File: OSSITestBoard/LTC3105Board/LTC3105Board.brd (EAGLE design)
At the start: 20.3 x 22.9 mm, 20 parts, among them U1 LT3105-MS

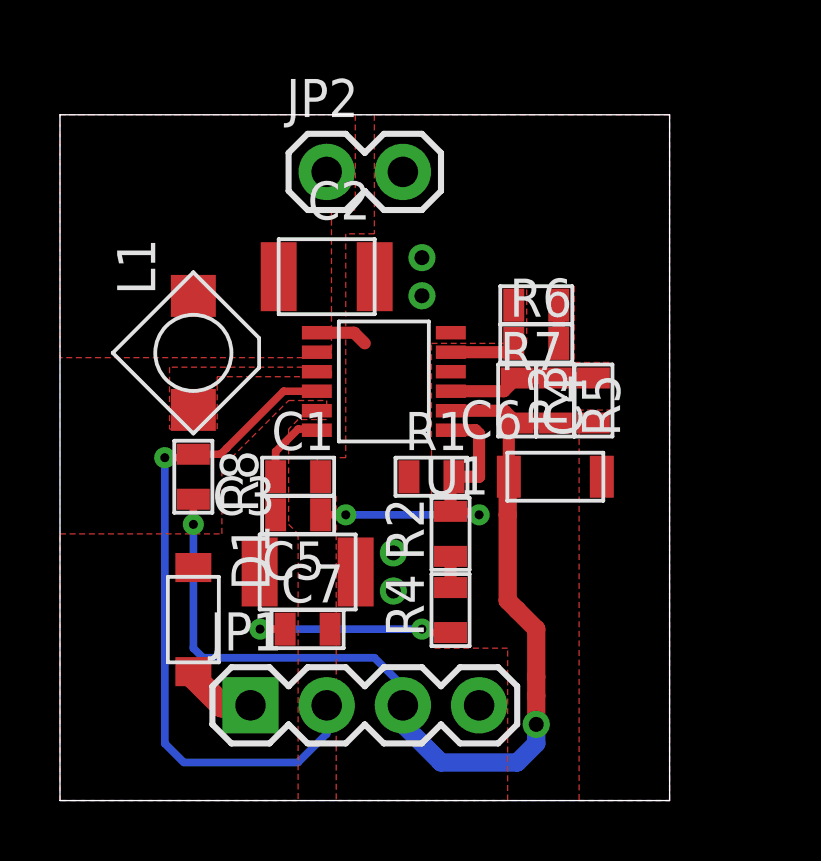
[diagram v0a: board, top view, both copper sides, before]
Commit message: LTC3105 board notes added
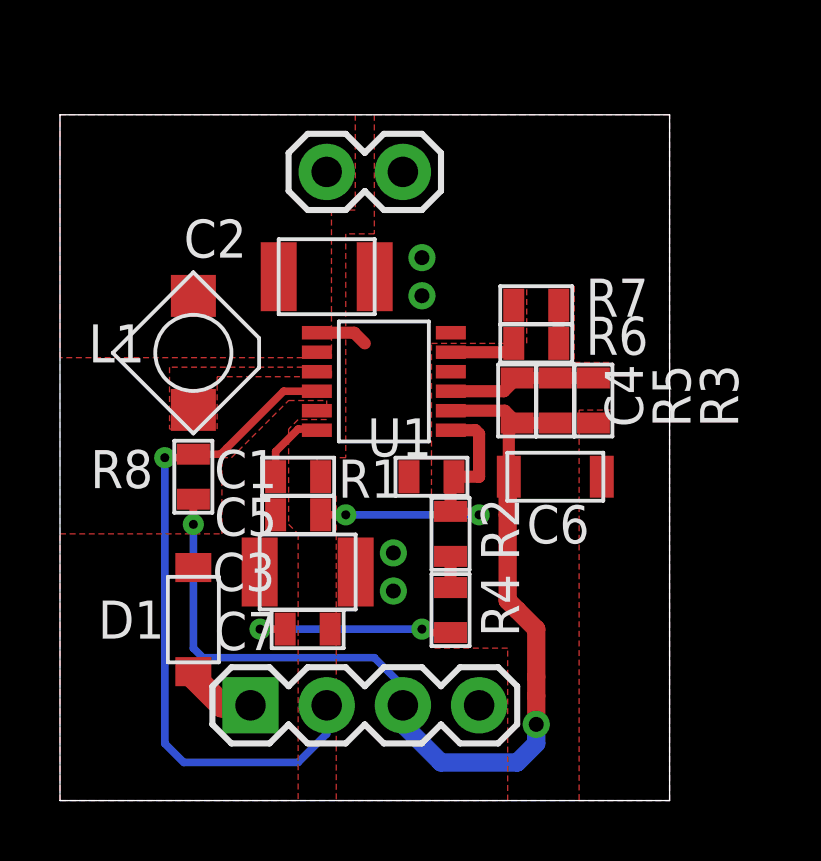
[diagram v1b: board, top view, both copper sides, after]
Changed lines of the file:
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@@
 <layer number="19" name="Unrouted" color="6" fill="1" visible="yes" active="yes"/>
 <layer number="20" name="Dimension" color="15" fill="1" visible="yes" active="yes"/>
-<layer number="21" name="tPlace" color="7" fill="1" visible="yes" active="yes"/>
+<layer number="21" name="tPlace" color="7" fill="1" visible="no" active="yes"/>
 <layer number="22" name="bPlace" color="7" fill="1" visible="no" active="yes"/>
-<layer number="23" name="tOrigins" color="15" fill="1" visible="yes" active="yes"/>
-<layer number="24" name="bOrigins" color="15" fill="1" visible="yes" active="yes"/>
-<layer number="25" name="tNames" color="7" fill="1" visible="no" active="yes"/>
-<layer number="26" name="bNames" color="7" fill="1" visible="no" active="yes"/>
+<layer number="23" name="tOrigins" color="15" fill="1" visible="no" active="yes"/>
+<layer number="24" name="bOrigins" color="15" fill="1" visible="no" active="yes"/>
+<layer number="25" name="tNames" color="7" fill="1" visible="yes" active="yes"/>
+<layer number="26" name="bNames" color="7" fill="1" visible="yes" active="yes"/>
 <layer number="27" name="tValues" color="7" fill="1" visible="no" active="yes"/>
 <layer number="28" name="bValues" color="7" fill="1" visible="no" active="yes"/>
-<layer number="29" name="tStop" color="7" fill="3" visible="yes" active="yes"/>
-<layer number="30" name="bStop" color="7" fill="6" visible="yes" active="yes"/>
+<layer number="29" name="tStop" color="7" fill="3" visible="no" active="yes"/>
+<layer number="30" name="bStop" color="7" fill="6" visible="no" active="yes"/>
 <layer number="31" name="tCream" color="7" fill="4" visible="no" active="yes"/>
 <layer number="32" name="bCream" color="7" fill="5" visible="no" active="yes"/>
@@
 <rectangle x1="0" y1="-1.27" x2="20.32" y2="21.59" layer="29"/>
 <rectangle x1="0" y1="-1.27" x2="20.32" y2="21.59" layer="30"/>
+<circle x="12.7" y="10.16" radius="0.3175" width="0.254" layer="48"/>
 </plain>
 <attributes>
@@
 <elements>
 <element name="U1" library="OSSI" package="MSOP-12-MS" value="LT3105-MS" x="10.795" y="12.7" smashed="yes" rot="R90">
-<attribute name="NAME" x="14.295" y="10.2" size="1.27" layer="25" font="vector" rot="R180"/>
+<attribute name="NAME" x="12.39" y="11.47" size="1.27" layer="25" font="vector" rot="R180"/>
 <attribute name="VALUE" x="14.295" y="16.2" size="1.27" layer="27" rot="R180"/>
 </element>
 <element name="L1" library="OSSI" package="CDRH3D18" value="10uH" x="4.445" y="13.6525" smashed="yes" rot="R270">
-<attribute name="NAME" x="1.905" y="17.4625" size="1.27" layer="25" font="vector" rot="R270"/>
+<attribute name="NAME" x="0.9525" y="13.335" size="1.27" layer="25" font="vector"/>
 <attribute name="VALUE" x="-3.175" y="16.1925" size="1.27" layer="27" rot="R270"/>
 </element>
 <element name="C1" library="OSSI" package="C0603(1608)" value="1uF" x="7.9375" y="9.525" smashed="yes">
-<attribute name="NAME" x="7.0485" y="10.414" size="1.27" layer="25" font="vector"/>
+<attribute name="NAME" x="5.1435" y="9.144" size="1.27" layer="25" font="vector"/>
 <attribute name="VALUE" x="7.0485" y="7.493" size="1.27" layer="27"/>
 </element>
 <element name="C2" library="OSSI" package="C1210-GCM32" value="10uF, 1210" x="8.89" y="16.1925" smashed="yes">
-<attribute name="NAME" x="8.255" y="18.0975" size="1.27" layer="25" font="vector"/>
+<attribute name="NAME" x="4.1275" y="16.8275" size="1.27" layer="25" font="vector"/>
 <attribute name="VALUE" x="5.715" y="13.0175" size="1.27" layer="27"/>
 </element>
 <element name="R1" library="OSSI" package="R0603(1608)" value="499k, 1%" x="12.3825" y="9.525" smashed="yes">
-<attribute name="NAME" x="11.4935" y="10.414" size="1.27" layer="25" font="vector"/>
+<attribute name="NAME" x="9.271" y="8.8265" size="1.27" layer="25" font="vector"/>
 <attribute name="VALUE" x="11.4935" y="7.493" size="1.27" layer="27"/>
 </element>
 <element name="R2" library="OSSI" package="R0603(1608)" value="392k, 1%" x="13.0175" y="7.62" smashed="yes" rot="R90">
-<attribute name="NAME" x="12.1285" y="6.731" size="1.27" layer="25" font="vector" rot="R90"/>
+<attribute name="NAME" x="15.3035" y="6.731" size="1.27" layer="25" font="vector" rot="R90"/>
 <attribute name="VALUE" x="15.0495" y="6.731" size="1.27" layer="27" rot="R90"/>
 </element>
 <element name="C4" library="OSSI" package="C0603(1608)" value="33pF" x="15.24" y="12.065" smashed="yes" rot="R270">
-<attribute name="NAME" x="16.129" y="12.954" size="1.27" layer="25" font="vector" rot="R270"/>
+<attribute name="NAME" x="19.431" y="11.176" size="1.27" layer="25" font="vector" rot="R90"/>
 <attribute name="VALUE" x="13.208" y="12.954" size="1.27" layer="27" rot="R270"/>
 </element>
 <element name="R3" library="OSSI" package="R0603(1608)" value="549k, 1%" x="17.78" y="12.065" smashed="yes" rot="R90">
-<attribute name="NAME" x="16.891" y="11.176" size="1.27" layer="25" font="vector" rot="R90"/>
+<attribute name="NAME" x="22.606" y="11.176" size="1.27" layer="25" font="vector" rot="R90"/>
 <attribute name="VALUE" x="19.812" y="11.176" size="1.27" layer="27" rot="R90"/>
 </element>
 <element name="R4" library="OSSI" package="R0603(1608)" value="750k, 1%" x="13.0175" y="5.08" smashed="yes" rot="R90">
-<attribute name="NAME" x="12.1285" y="4.191" size="1.27" layer="25" font="vector" rot="R90"/>
+<attribute name="NAME" x="15.3035" y="4.191" size="1.27" layer="25" font="vector" rot="R90"/>
 <attribute name="VALUE" x="15.0495" y="4.191" size="1.27" layer="27" rot="R90"/>
 </element>
 <element name="C5" library="OSSI" package="C0603(1608)" value="33pF" x="7.9375" y="8.255" smashed="yes" rot="R180">
-<attribute name="NAME" x="8.8265" y="7.366" size="1.27" layer="25" font="vector" rot="R180"/>
+<attribute name="NAME" x="5.1435" y="7.5565" size="1.27" layer="25" font="vector"/>
 <attribute name="VALUE" x="8.8265" y="10.287" size="1.27" layer="27" rot="R180"/>
 </element>
 <element name="R5" library="OSSI" package="R0603(1608)" value="1.1M, 1%" x="16.51" y="12.065" smashed="yes" rot="R270">
-<attribute name="NAME" x="17.399" y="12.954" size="1.27" layer="25" font="vector" rot="R270"/>
+<attribute name="NAME" x="21.0185" y="11.176" size="1.27" layer="25" font="vector" rot="R90"/>
 <attribute name="VALUE" x="14.478" y="12.954" size="1.27" layer="27" rot="R270"/>
 </element>
 <element name="R6" library="OSSI" package="R0603(1608)" value="TBD" x="15.875" y="13.97" smashed="yes">
-<attribute name="NAME" x="14.986" y="14.859" size="1.27" layer="25" font="vector"/>
+<attribute name="NAME" x="17.526" y="13.589" size="1.27" layer="25" font="vector"/>
 <attribute name="VALUE" x="14.986" y="11.938" size="1.27" layer="27"/>
 </element>
 <element name="R7" library="OSSI" package="R0603(1608)" value="TBD" x="15.875" y="15.24" smashed="yes" rot="R180">
-<attribute name="NAME" x="16.764" y="14.351" size="1.27" layer="25" font="vector" rot="R180"/>
+<attribute name="NAME" x="17.526" y="14.859" size="1.27" layer="25" font="vector"/>
 <attribute name="VALUE" x="16.764" y="17.272" size="1.27" layer="27" rot="R180"/>
 </element>
 <element name="R8" library="OSSI" package="R0603(1608)" value="100k" x="4.445" y="9.525" smashed="yes" rot="R270">
-<attribute name="NAME" x="5.334" y="10.414" size="1.27" layer="25" font="vector" rot="R270"/>
+<attribute name="NAME" x="1.016" y="9.144" size="1.27" layer="25" font="vector"/>
 <attribute name="VALUE" x="2.413" y="10.414" size="1.27" layer="27" rot="R270"/>
 </element>
 <element name="C6" library="OSSI" package="C1206-GCM31" value="4.7uF, 1206" x="16.51" y="9.525" smashed="yes">
-<attribute name="NAME" x="13.335" y="10.795" size="1.27" layer="25" font="vector"/>
+<attribute name="NAME" x="15.5575" y="7.3025" size="1.27" layer="25" font="vector"/>
 <attribute name="VALUE" x="13.335" y="6.985" size="1.27" layer="27"/>
 </element>
 <element name="C3" library="OSSI" package="C1210-GCM32" value="10uF, 1210" x="8.255" y="6.35" smashed="yes">
-<attribute name="NAME" x="5.08" y="8.255" size="1.27" layer="25" font="vector"/>
+<attribute name="NAME" x="5.08" y="5.715" size="1.27" layer="25" font="vector"/>
 <attribute name="VALUE" x="5.08" y="3.175" size="1.27" layer="27"/>
 </element>
 <element name="C7" library="OSSI" package="C0603(1608)" value="1uF" x="8.255" y="4.445" smashed="yes">
-<attribute name="NAME" x="7.366" y="5.334" size="1.27" layer="25" font="vector"/>
+<attribute name="NAME" x="5.1435" y="3.7465" size="1.27" layer="25" font="vector"/>
 <attribute name="VALUE" x="7.366" y="2.413" size="1.27" layer="27"/>
 </element>
-<element name="JP1" library="OSSI" package="1X04" value="" x="6.35" y="1.905"/>
-<element name="JP2" library="OSSI" package="1X02" value="" x="8.89" y="19.685"/>
-<element name="D1" library="OSSI" package="SOD-123" value="STPS0520Z" x="4.445" y="4.7625" rot="R270"/>
+<element name="JP1" library="OSSI" package="1X04" value="" x="6.35" y="1.905" smashed="yes">
+<attribute name="VALUE" x="5.08" y="-1.27" size="1.27" layer="27"/>
+</element>
+<element name="JP2" library="OSSI" package="1X02" value="" x="8.89" y="19.685" smashed="yes">
+<attribute name="VALUE" x="7.62" y="16.51" size="1.27" layer="27"/>
+</element>
+<element name="D1" library="OSSI" package="SOD-123" value="STPS0520Z" x="4.445" y="4.7625" smashed="yes" rot="R270">
+<attribute name="NAME" x="1.27" y="4.1275" size="1.27" layer="25" font="vector"/>
+<attribute name="VALUE" x="1.905" y="7.9375" size="1.27" layer="27" rot="R270"/>
+</element>
 </elements>
 <signals>
